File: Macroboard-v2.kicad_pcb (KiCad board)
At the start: 2 copper layers, 76.2 x 88.4 mm, 14 parts, among them Q2 Q_NPN_BEC, SW5 SW_DIP_x01, SW6 SW_DIP_x01, SW7 SW_DIP_x01, SW8 SW_DIP_x01, U1 XIAO-RP2040-DIP

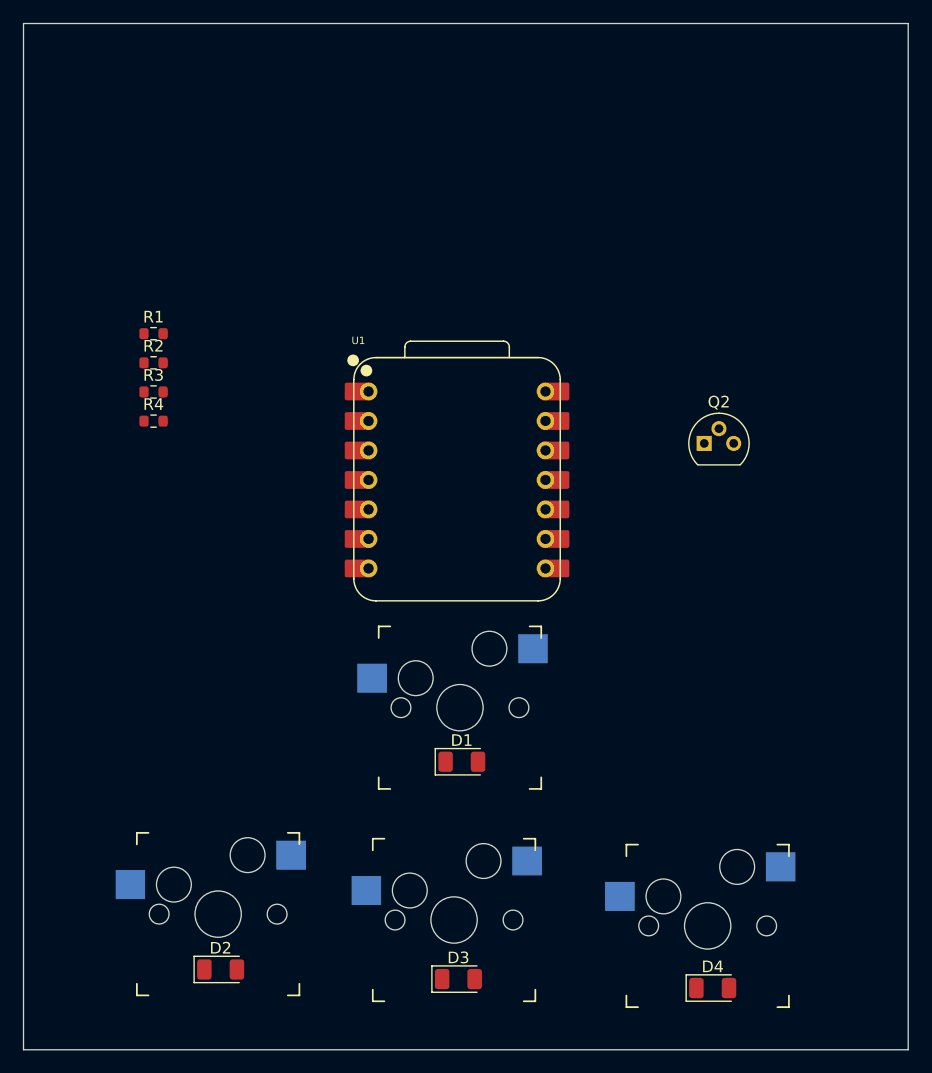
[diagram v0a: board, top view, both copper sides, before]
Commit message: Schemetics and PCB Desing completed . T- 1756 -20250522
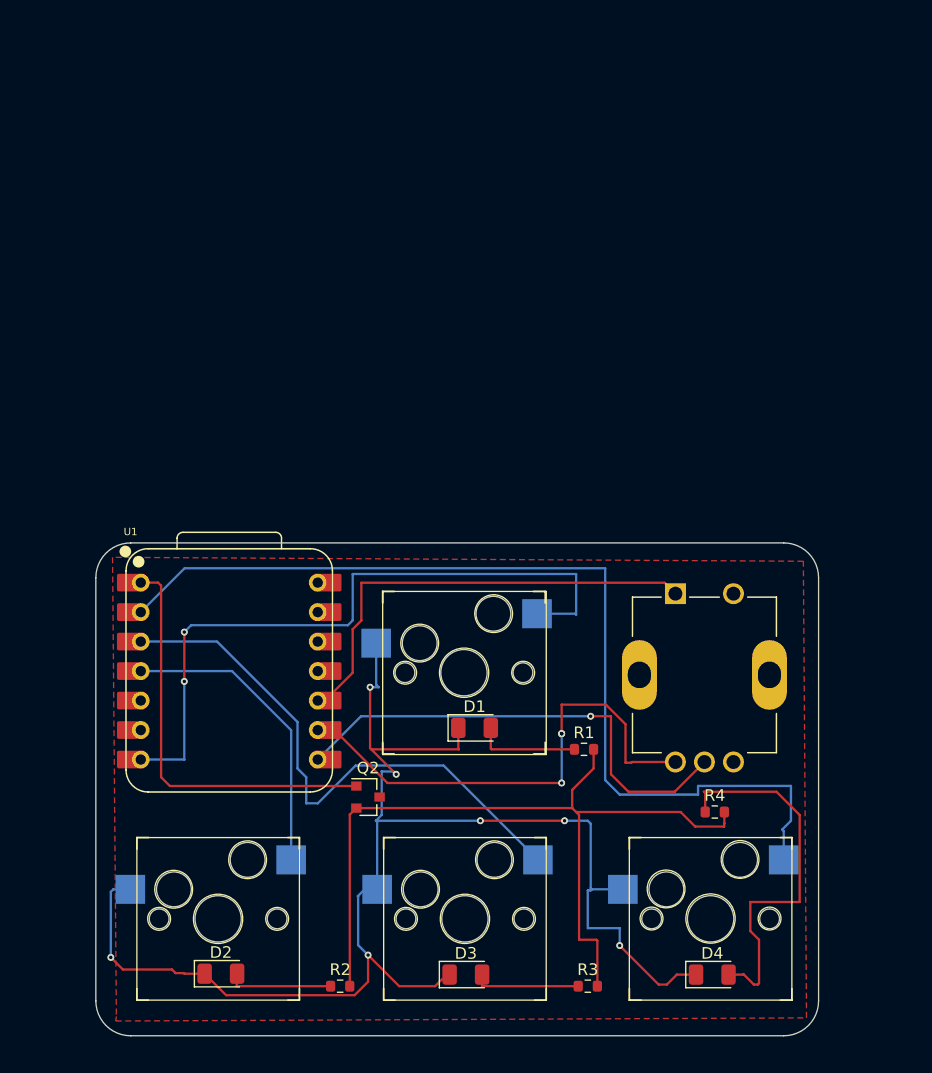
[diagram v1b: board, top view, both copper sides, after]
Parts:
- added S2: PEC12R-4015F-S0024, PEC12R-4015F-S0024 Rotary Encoder:XDCR_PEC12R-4015F-S0024, F.Cu at (147.6, 93.2)
- Q2: footprint Package_TO_SOT_THT:TO-92 -> Transistor:SOT-23
- moved R3 63.4 mm to (137.5, 120.0)
- moved R4 58.9 mm to (148.4, 105.0)
- moved R2 56.0 mm to (116.2, 120.0)
- moved R1 51.5 mm to (137.2, 99.6)
- moved Q2 42.0 mm to (118.6, 103.7)
- moved U1 25.6 mm to (106.6, 92.9)
- moved D1 3.12 mm to (127.8, 97.8)
- moved SW5 3.03 mm to (126.8, 93.0)
- moved D4 1.16 mm to (148.2, 119.0)
- moved SW7 0.94 mm to (126.9, 114.2)
- moved D3 0.75 mm to (127.0, 119.0)
- moved SW8 0.66 mm to (148.1, 114.2)
- moved SW6 0.41 mm to (105.7, 114.2)
- moved D2 0.37 mm to (105.9, 118.9)
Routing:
- net GND: track 0.00 -> 126.3 mm, vias 0 -> 7
- net Net-(U1-GPIO27/ADC1/A1): track 0.00 -> 83.8 mm
- net Net-(Q2-E): track 0.00 -> 71.6 mm
- net Net-(U1-GPIO0/TX): track 0.00 -> 59.8 mm, vias 0 -> 2
- net Net-(U1-GPIO28/ADC2/A2): track 0.00 -> 48.4 mm
- net Net-(S2-CHANNEL_A): track 0.00 -> 43.5 mm, vias 0 -> 3
- net Net-(S2-COMMON): track 0.00 -> 41.5 mm, vias 0 -> 1
- net Net-(U1-GPIO4/MISO): track 0.00 -> 39.5 mm
- net Net-(Q2-B): track 0.00 -> 35.5 mm
- net Net-(D4-A): track 0.00 -> 33.0 mm
- net Net-(U1-GPIO29/ADC3/A3): track 0.00 -> 26.2 mm
- net Net-(D2-A): track 0.00 -> 9.53 mm
- net Net-(D3-A): track 0.00 -> 9.35 mm
- net Net-(D1-A): track 0.00 -> 9.02 mm
- added copper zone on F.Cu, net GND
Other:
- board size 76.2 x 88.4 mm -> 62.2 x 42.5 mm
